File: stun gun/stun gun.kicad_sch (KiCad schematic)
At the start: 14 parts, among them J1 Power, J2 Digital/PWM, J3 Analog, J4 Digital/PWM, T1 Transformer_1P_1S, U1 LCD-016N002L, U2 Magnetic Sensor

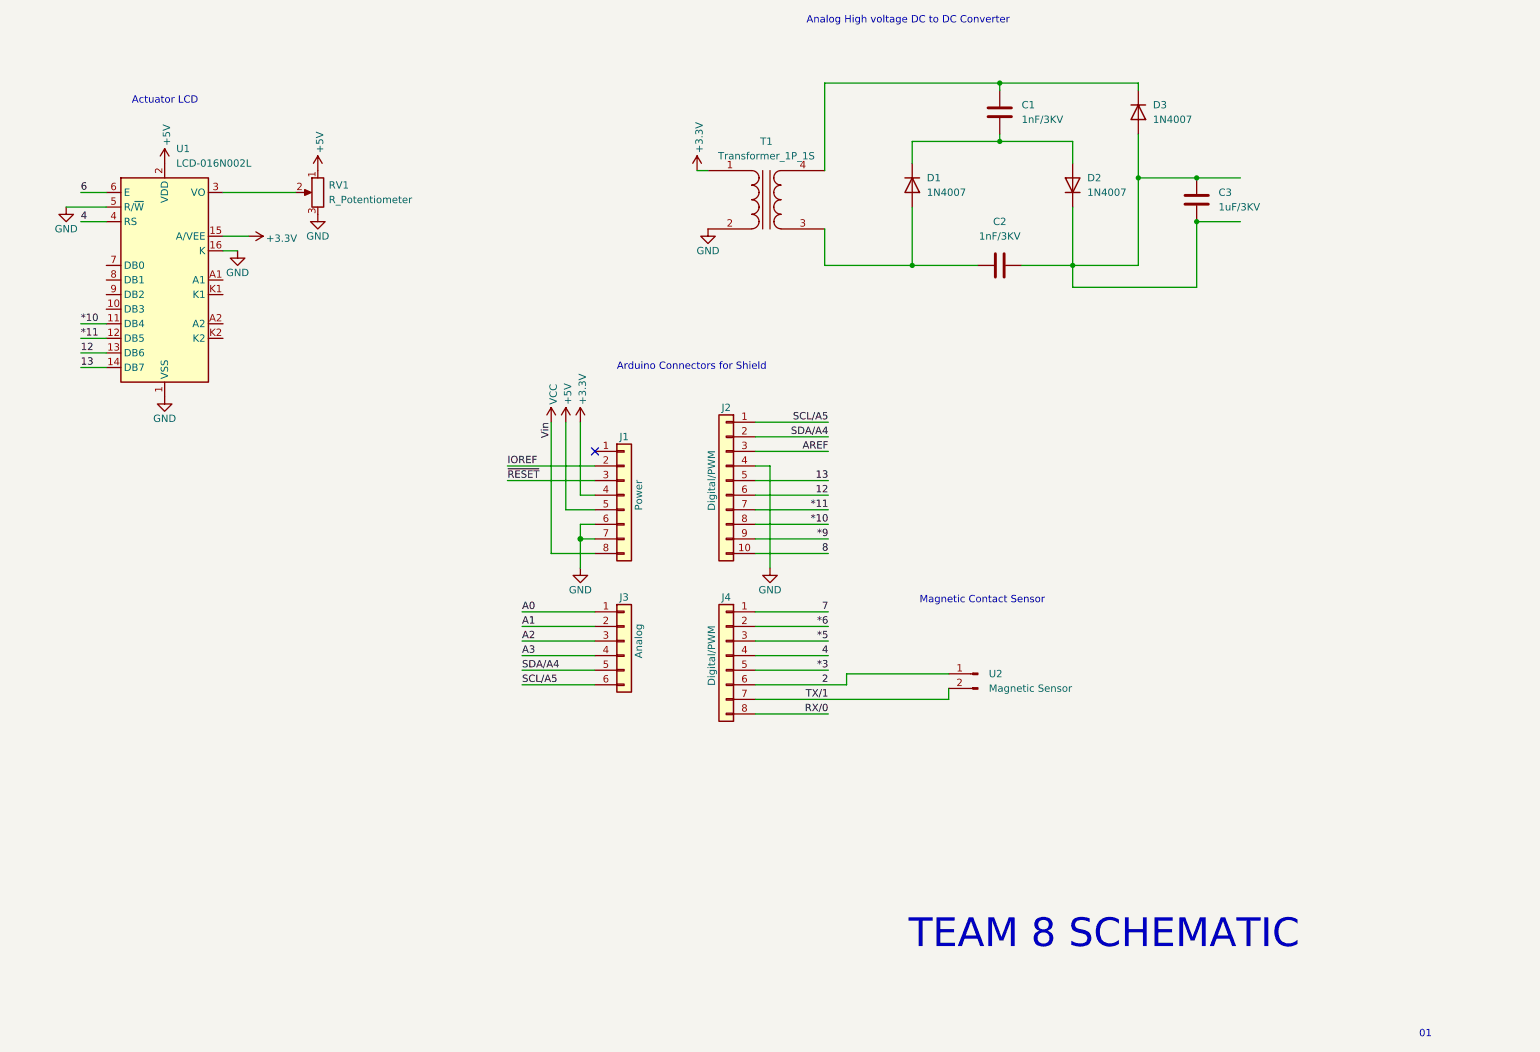
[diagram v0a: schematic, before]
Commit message: Add files via upload
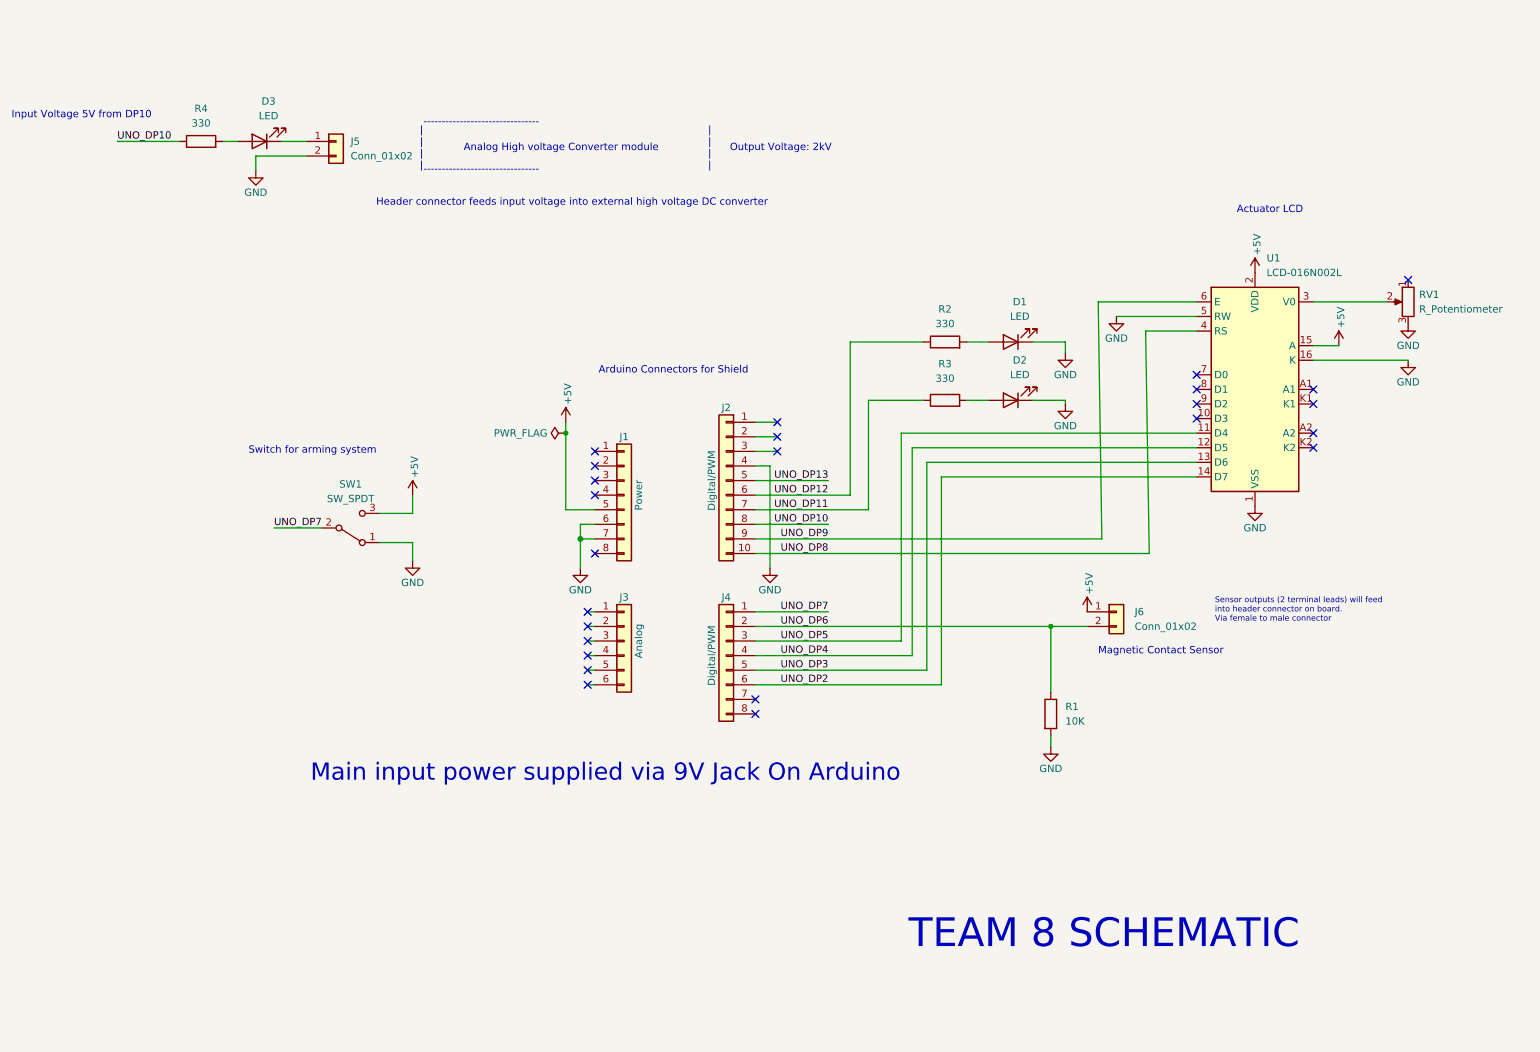
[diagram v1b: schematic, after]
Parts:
- removed C1, C2: 1nF/3KV, Capacitor_SMD:C_0805_2012Metric, symbol Device:C
- removed C3: 1uF/3KV, Capacitor_SMD:C_0805_2012Metric, symbol Device:C
- removed D1, D2, D3: 1N4007, Diode_THT:D_DO-41_SOD81_P7.62mm_Horizontal, symbol Device:D
- removed T1: Transformer_1P_1S, Transformer_THT:Transformer_NF_ETAL_1-1_P1200, symbol Device:Transformer_1P_1S
- removed U2: Magnetic Sensor, symbol Connector:Conn_01x02_Male
- added D1, D2, D3: LED, LED_THT:LED_D3.0mm, symbol Device:LED
- added J5, J6: Conn_01x02, Connector_PinHeader_2.54mm:PinHeader_1x02_P2.54mm_Vertical, symbol Connector_Generic:Conn_01x02
- added R1: 10K, Resistor_SMD:R_0805_2012Metric, symbol Device:R
- added R2, R3, R4: 330, Resistor_SMD:R_0805_2012Metric, symbol Device:R
- added SW1: SW_SPDT, slideswitch:EG1218, symbol Switch:SW_SPDT
- J3: now left out of the parts list
- RV1: footprint Potentiometer_THT:Potentiometer_Piher_T-16L_Single_Vertical_Hole -> trimmer:TRIM_3362P-1-505LF
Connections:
- net 6 is gone; now on net UNO_DP9: U1.6 (E)
- net +5V: now also U1.15 (A), J6.1 (Pin_1), SW1.3 (C); no longer RV1.1
- net GND: now also D1.1 (K), D2.1 (K), J5.2 (Pin_2), R1.2, SW1.1 (A)
- net *10 renamed UNO_DP10
- net UNO_DP10: now also R4.1; no longer U1.11 (DB4)
- net *11 renamed UNO_DP11
- net UNO_DP11: now also R3.1; no longer U1.12 (DB5)
- net *3 renamed UNO_DP3
- net UNO_DP3: now also U1.13 (D6)
- net *5 renamed UNO_DP5
- net UNO_DP5: now also U1.11 (D4)
- net *6 renamed UNO_DP6
- net UNO_DP6: now also J6.2 (Pin_2), R1.1
- net *9 renamed UNO_DP9
- net +3V3: no longer names the net of J1.4 (Pin_4)
- net +3V3: no longer U1.15 (A/VEE)
- net 12 renamed UNO_DP12
- net UNO_DP12: now also R2.1; no longer U1.13 (DB6)
- net 13 renamed UNO_DP13
- net UNO_DP13: no longer U1.14 (DB7)
- net 2 renamed UNO_DP2
- net UNO_DP2: now also U1.14 (D7)
- net 4 renamed UNO_DP4
- net UNO_DP4: now also U1.12 (D5); no longer U1.4 (RS)
- net 7 renamed UNO_DP7
- net UNO_DP7: now also SW1.2 (B)
- net 8 renamed UNO_DP8
- net UNO_DP8: now also U1.4 (RS)
- net A0: no longer names the net of J3.1 (Pin_1)
- net A1: no longer names the net of J3.2 (Pin_2)
- net A2: no longer names the net of J3.3 (Pin_3)
- net A3: no longer names the net of J3.4 (Pin_4)
- net AREF: no longer names the net of J2.3 (Pin_3)
- net IOREF: no longer names the net of J1.2 (Pin_2)
- net RX/0: no longer names the net of J4.8 (Pin_8)
- net SCL/A5: no longer names the net of J2.1 (Pin_1)
- net SCL/A5: no longer J3.6 (Pin_6)
- net SDA/A4: no longer names the net of J2.2 (Pin_2)
- net SDA/A4: no longer J3.5 (Pin_5)
- net TX/1: no longer names the net of J4.7 (Pin_7)
- net VCC: no longer names the net of J1.8 (Pin_8)
- net ~{RESET}: no longer names the net of J1.3 (Pin_3)
- new net: D2.2 (A), R3.2
- new net: D1.2 (A), R2.2
- new net: D3.1 (K), J5.1 (Pin_1)
- new net: D3.2 (A), R4.2
- no-connect marks 1 -> 25
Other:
- note added: "--------------------------------"
- note added: "Analog High voltage Converter module"
- note added: "Header connector feeds input voltage into external high voltage DC converter"
- note added: "Input Voltage 5V from DP10"
- note added: "Main input power supplied via 9V Jack On Arduino"
- note added: "Output Voltage: 2kV"
- note added: "Sensor outputs (2 terminal leads) will feed into header connector on board. Via female to male connector"
- note added: "Switch for arming system"
- note added: "| | | |"
- note removed: "01"
- note removed: "Analog High voltage DC to DC Converter"
- moved on the sheet: RV1, U1
